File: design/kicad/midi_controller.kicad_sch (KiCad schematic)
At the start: 5 parts, among them J1 Conn_01x16_Socket, J2 Conn_01x25_Socket, J3 Conn_01x25_Socket, U1 CD74HC4067SM

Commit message: Refactor code structure for improved readability and maintainability
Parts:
- removed J1: Conn_01x16_Socket, Connector_PinSocket_2.54mm:PinSocket_1x16_P2.54mm_Vertical, symbol Connector:Conn_01x16_Socket
- removed J2, J3: Conn_01x25_Socket, Connector_PinSocket_2.54mm:PinSocket_1x25_P2.54mm_Vertical, symbol Connector:Conn_01x25_Socket
- removed U1: CD74HC4067SM, Package_SO:SSOP-24_5.3x8.2mm_P0.65mm, symbol 74xx:CD74HC4067SM
- added D1: MIDI_Display_MSP2807, midi_controller:MSP2807_ILI9341_Display, symbol midi_controller:MIDI_Display_MSP2807
- added ENC_MECH1, ENC_MECH2, ENC_MECH3, ENC_MECH4, ENC_MECH5, ENC_MECH6, ENC_MECH7, ENC_MECH8, ENC_MECH9: MIDI_Encoder_PEC11R, midi_controller:PEC11R4220FS0024, symbol midi_controller:MIDI_Encoder_PEC11R
- added ENC_OPT1: MIDI_Encoder_E38S6G5_Optical, midi_controller:E38S6G5_Optical_Encoder, symbol midi_controller:MIDI_Encoder_E38S6G5_Optical
- added J1, J2: Conn_01x24_Socket, symbol Connector:Conn_01x24_Socket
- added R1: R, Resistor_THT:R_Axial_DIN0204_L3.6mm_D1.6mm_P7.62mm_Horizontal, symbol Device:R
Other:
- moved on the sheet: MCU1

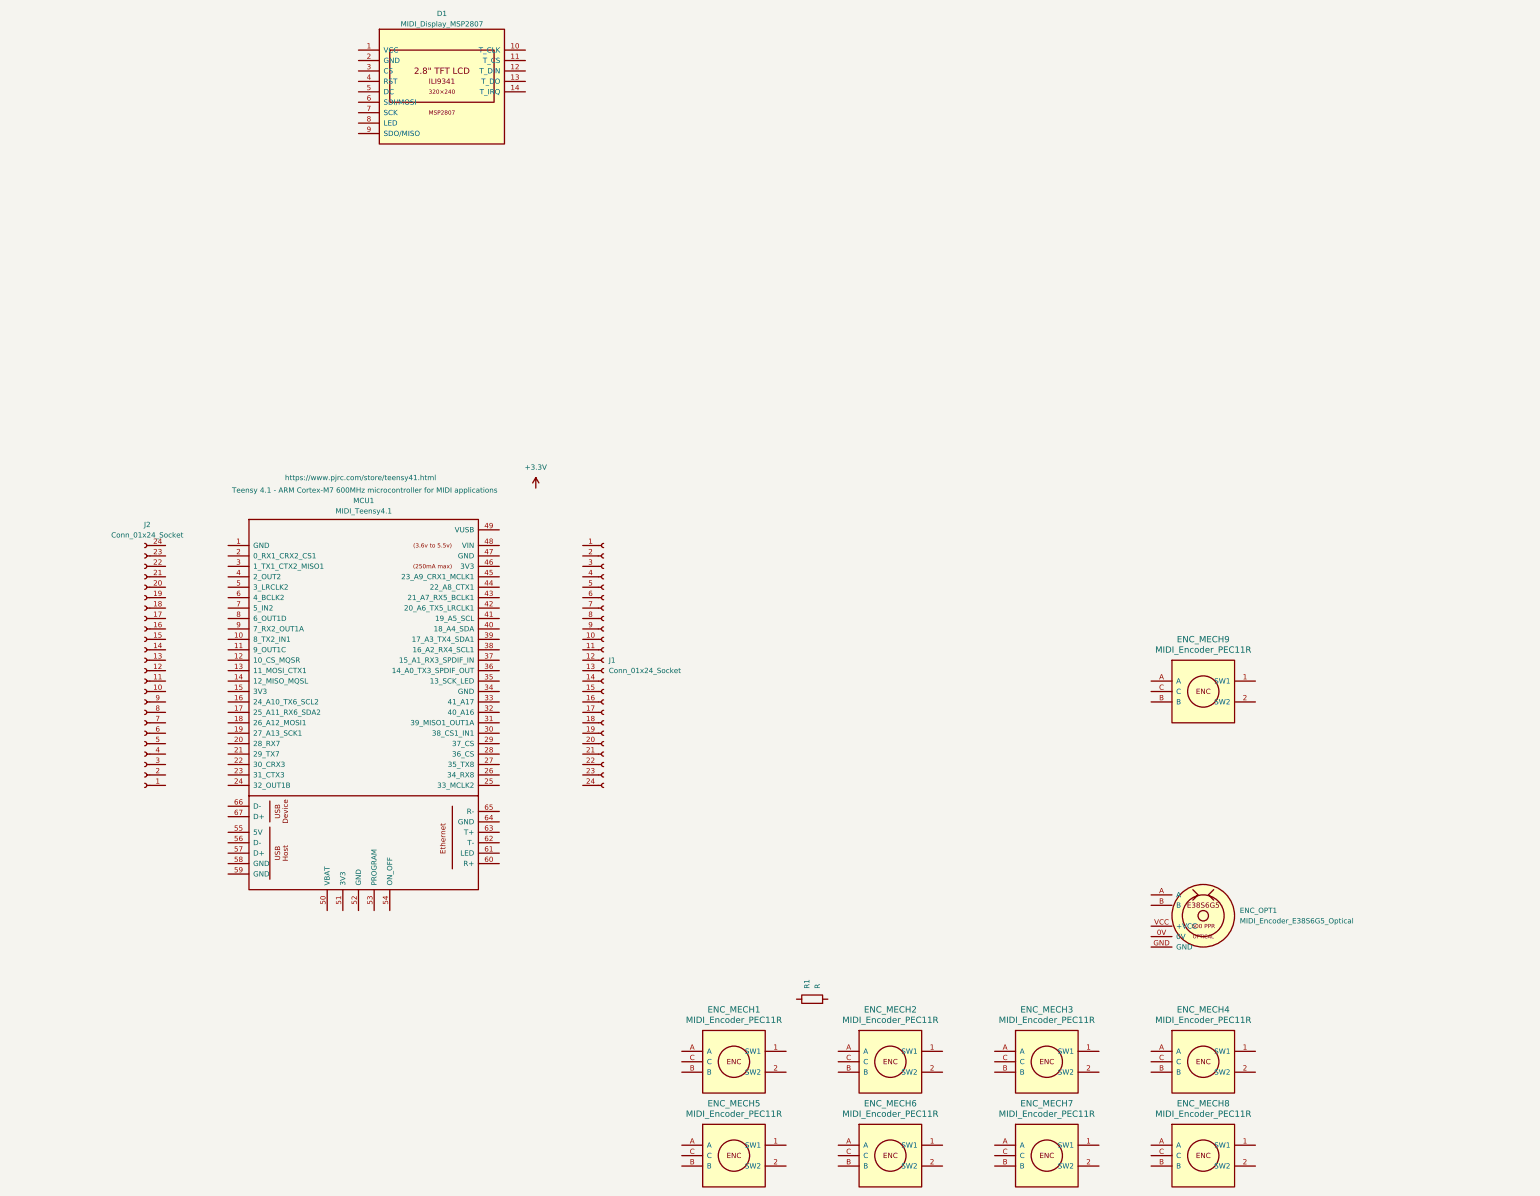
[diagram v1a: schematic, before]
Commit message: Refactor code structure for improved readability and maintainability
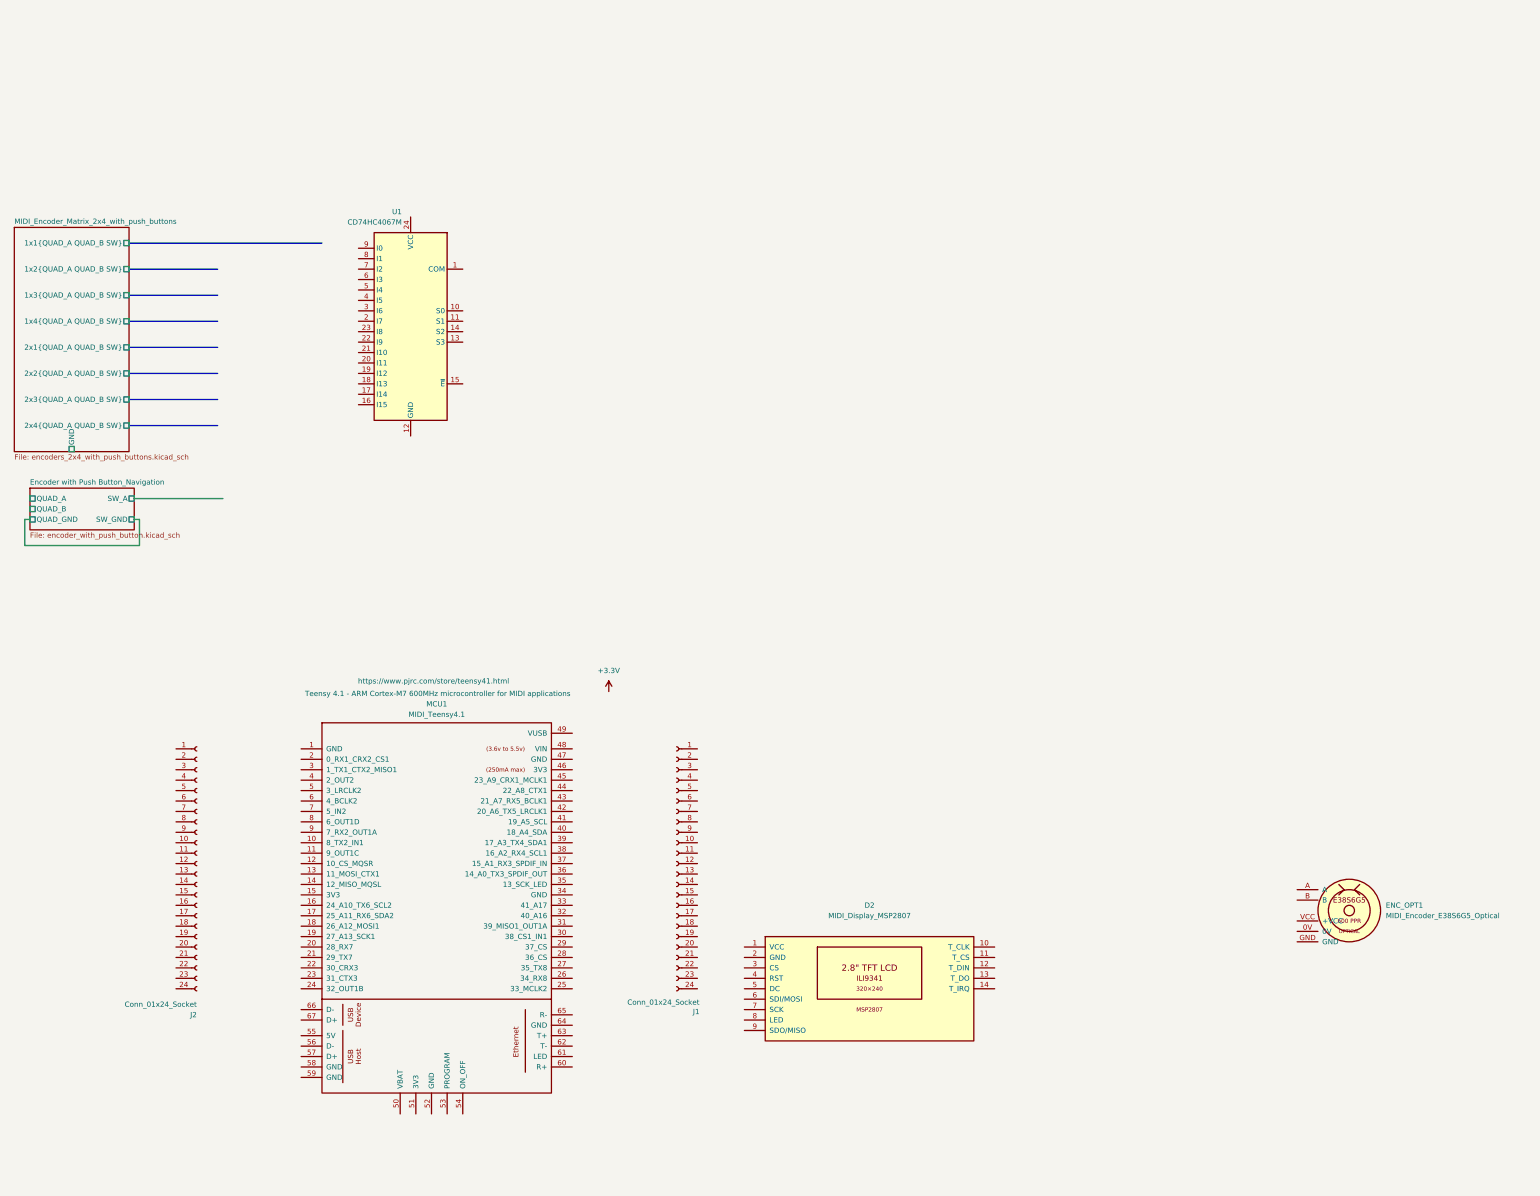
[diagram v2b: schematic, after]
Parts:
- removed D1: MIDI_Display_MSP2807, midi_controller:MSP2807_ILI9341_Display, symbol midi_controller:MIDI_Display_MSP2807
- removed ENC_MECH1, ENC_MECH2, ENC_MECH3, ENC_MECH4, ENC_MECH5, ENC_MECH6, ENC_MECH7, ENC_MECH8, ENC_MECH9: MIDI_Encoder_PEC11R, midi_controller:PEC11R4220FS0024, symbol midi_controller:MIDI_Encoder_PEC11R
- removed R1: R, Resistor_THT:R_Axial_DIN0204_L3.6mm_D1.6mm_P7.62mm_Horizontal, symbol Device:R
- added D2: MIDI_Display_MSP2807, midi_controller:MSP2807_ILI9341_Display, symbol midi_controller:MIDI_Display_MSP2807
- added U1: CD74HC4067M, Package_SO:SSOP-24_5.3x8.2mm_P0.65mm, symbol 74xx:CD74HC4067M
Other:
- added sheet Encoder with Push Button_Navigation (encoder_with_push_button.kicad_sch)
- added sheet MIDI_Encoder_Matrix_2x4_with_push_buttons (encoders_2x4_with_push_buttons.kicad_sch)
- moved on the sheet: ENC_OPT1, J1, J2, MCU1

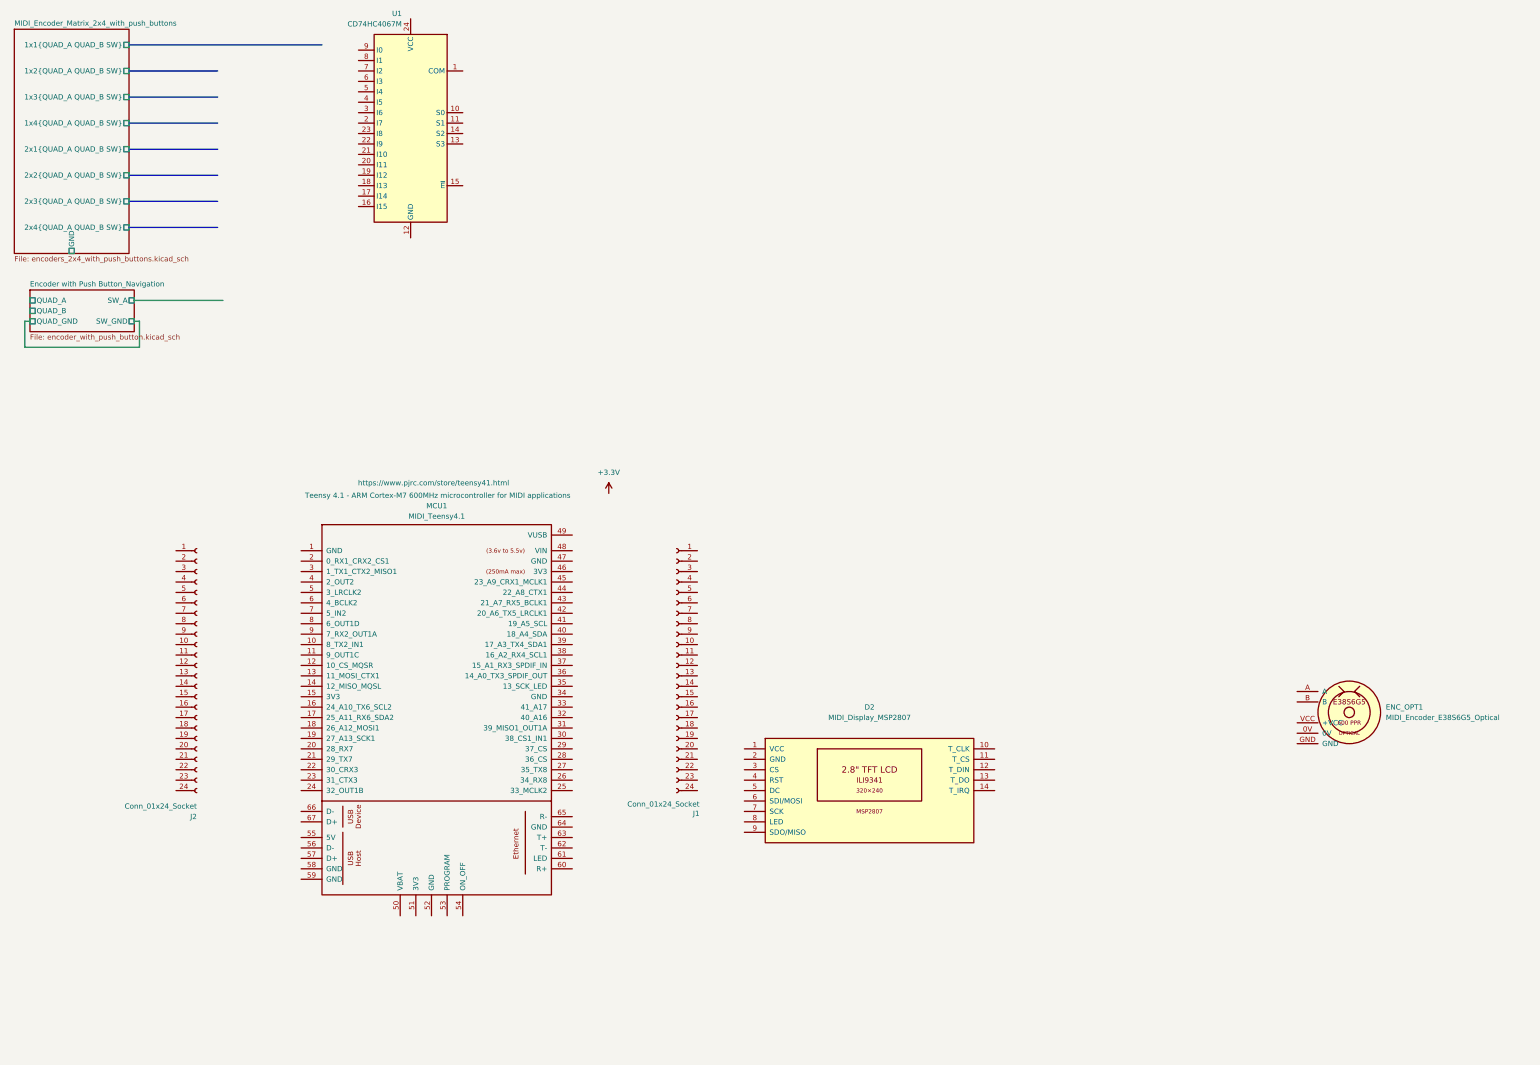
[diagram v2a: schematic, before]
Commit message: Refactor code structure for improved readability and maintainability
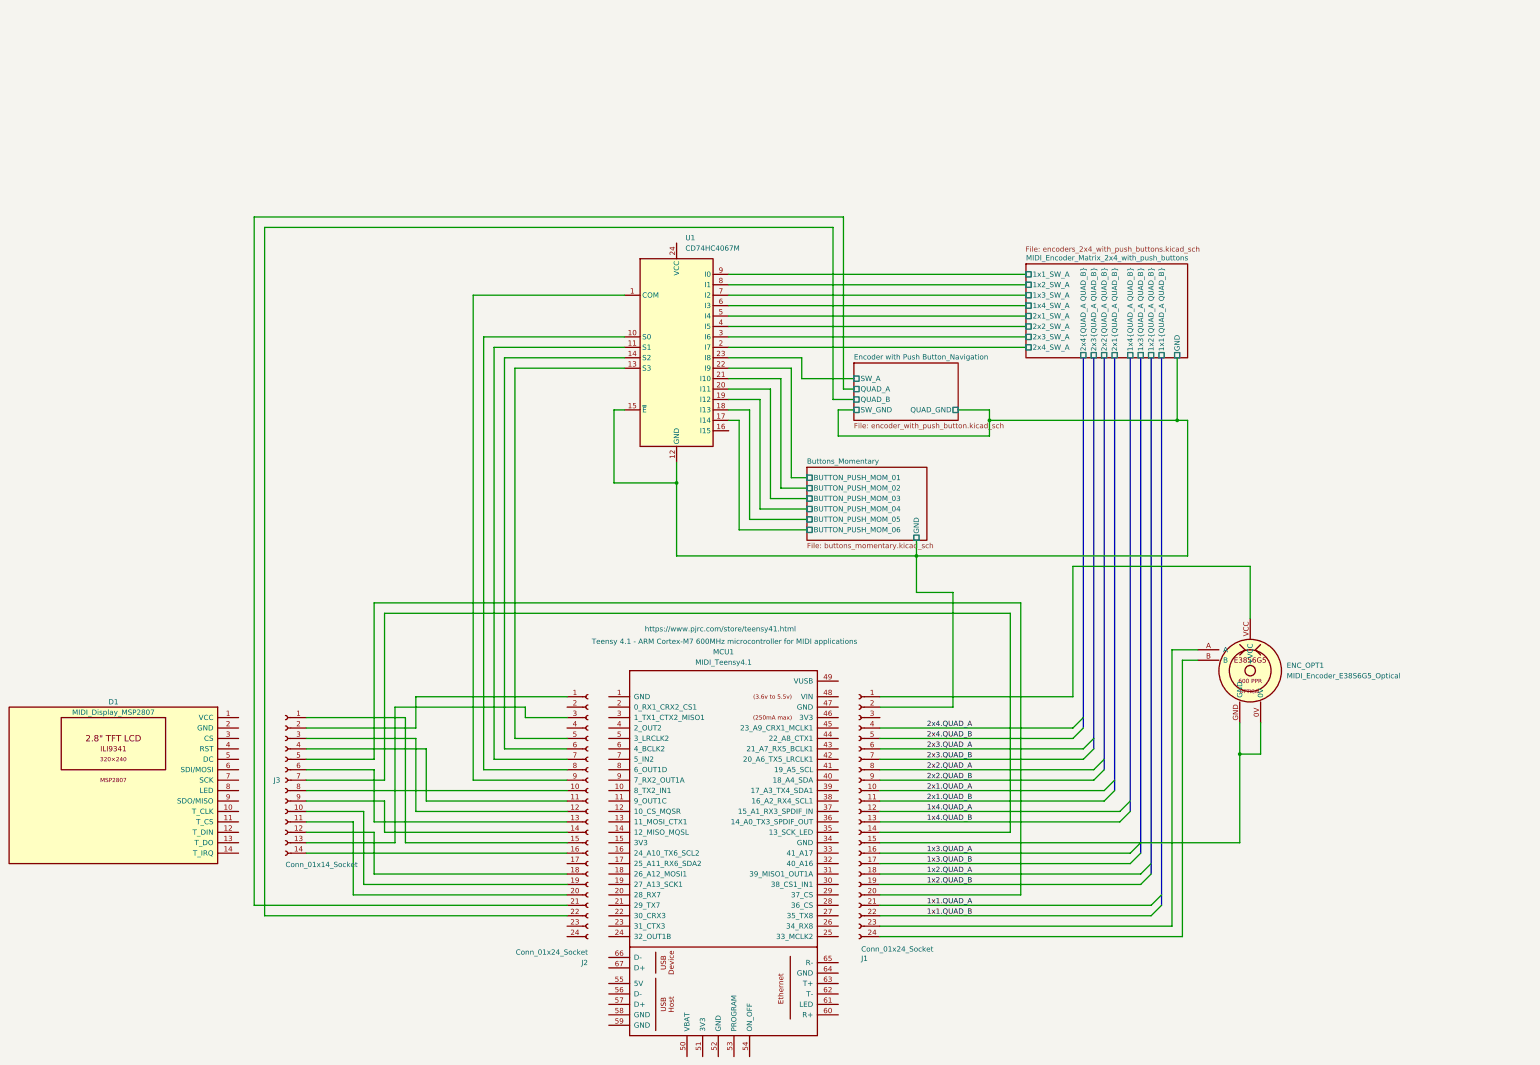
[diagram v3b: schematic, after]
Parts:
- added J3: Conn_01x14_Socket, Connector_PinSocket_2.54mm:PinSocket_1x14_P2.54mm_Vertical, symbol Connector:Conn_01x14_Socket
- J1, J2: footprint (none) -> Connector_PinSocket_2.54mm:PinSocket_1x24_P2.54mm_Vertical
- U1: footprint Package_SO:SSOP-24_5.3x8.2mm_P0.65mm -> Package_SO:SOIC-24W_7.5x15.4mm_P1.27mm
- renumbered D2 to D1
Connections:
- net Encoder with Push Button_Navigation/QUAD_A: now also J2.21 (Pin_21)
- net Encoder with Push Button_Navigation/QUAD_B: now also J2.22 (Pin_22)
- net Encoder with Push Button_Navigation/SW_A: now also U1.23 (I8)
- net at J1.1 (Pin_1): now also ENC_OPT1.VCC (+VCC)
- net 2x1.QUAD_A: now reaches J1.10 (Pin_10)
- net 2x1.QUAD_B: now reaches J1.11 (Pin_11)
- net 1x4.QUAD_A: now reaches J1.12 (Pin_12)
- net 1x4.QUAD_B: now reaches J1.13 (Pin_13)
- net at J1.14 (Pin_14): now also J3.7 (Pin_7)
- net at J1.15 (Pin_15): now also ENC_OPT1.0V, ENC_OPT1.GND
- net 1x3.QUAD_A: now reaches J1.16 (Pin_16)
- net 1x3.QUAD_B: now reaches J1.17 (Pin_17)
- net 1x2.QUAD_A: now reaches J1.18 (Pin_18)
- net 1x2.QUAD_B: now reaches J1.19 (Pin_19)
- net Buttons_Momentary/GND: now reaches J1.2 (Pin_2)
- net Buttons_Momentary/GND: now also U1.12 (GND), U1.15 (~{E})
- net at J1.20 (Pin_20): now also J3.5 (Pin_5)
- net 1x1.QUAD_A: now reaches J1.21 (Pin_21)
- net 1x1.QUAD_B: now reaches J1.22 (Pin_22)
- net at J1.23 (Pin_23): now also ENC_OPT1.A
- net at J1.24 (Pin_24): now also ENC_OPT1.B
- net 2x4.QUAD_A: now reaches J1.4 (Pin_4)
- net 2x4.QUAD_B: now reaches J1.5 (Pin_5)
- net 2x3.QUAD_A: now reaches J1.6 (Pin_6)
- net 2x3.QUAD_B: now reaches J1.7 (Pin_7)
- net 2x2.QUAD_A: now reaches J1.8 (Pin_8)
- net 2x2.QUAD_B: now reaches J1.9 (Pin_9)
- net at U1.1 (COM): now also J2.9 (Pin_9)
- net at U1.10 (S0): now also J2.8 (Pin_8)
- net at U1.11 (S1): now also J2.7 (Pin_7)
- net at U1.13 (S3): now also J2.5 (Pin_5)
- net at U1.14 (S2): now also J2.6 (Pin_6)
- net Buttons_Momentary/BUTTON_PUSH_MOM_06: now reaches U1.17 (I14)
- net Buttons_Momentary/BUTTON_PUSH_MOM_05: now reaches U1.18 (I13)
- net Buttons_Momentary/BUTTON_PUSH_MOM_04: now reaches U1.19 (I12)
- net MIDI_Encoder_Matrix_2x4_with_push_buttons/2x4_SW_A: now reaches U1.2 (I7)
- net Buttons_Momentary/BUTTON_PUSH_MOM_03: now reaches U1.20 (I11)
- net Buttons_Momentary/BUTTON_PUSH_MOM_02: now reaches U1.21 (I10)
- net Buttons_Momentary/BUTTON_PUSH_MOM_01: now reaches U1.22 (I9)
- net MIDI_Encoder_Matrix_2x4_with_push_buttons/2x3_SW_A: now reaches U1.3 (I6)
- net MIDI_Encoder_Matrix_2x4_with_push_buttons/2x2_SW_A: now reaches U1.4 (I5)
- net MIDI_Encoder_Matrix_2x4_with_push_buttons/2x1_SW_A: now reaches U1.5 (I4)
- net MIDI_Encoder_Matrix_2x4_with_push_buttons/1x4_SW_A: now reaches U1.6 (I3)
- net MIDI_Encoder_Matrix_2x4_with_push_buttons/1x3_SW_A: now reaches U1.7 (I2)
- net MIDI_Encoder_Matrix_2x4_with_push_buttons/1x2_SW_A: now reaches U1.8 (I1)
- net MIDI_Encoder_Matrix_2x4_with_push_buttons/1x1_SW_A: now reaches U1.9 (I0)
- net at J2.1 (Pin_1): now also J3.2 (Pin_2)
- net at J2.10 (Pin_10): now also J3.8 (Pin_8)
- net at J2.11 (Pin_11): now also J3.4 (Pin_4)
- net at J2.12 (Pin_12): now also J3.3 (Pin_3)
- net at J2.13 (Pin_13): now also J3.6 (Pin_6)
- net at J2.14 (Pin_14): now also J3.9 (Pin_9)
- net at J2.15 (Pin_15): now also J3.1 (Pin_1)
- net at J2.16 (Pin_16): now also J3.14 (Pin_14)
- net at J2.18 (Pin_18): now also J3.12 (Pin_12)
- net at J2.19 (Pin_19): now also J3.10 (Pin_10)
- net at J2.20 (Pin_20): now also J3.11 (Pin_11)
- net at J2.3 (Pin_3): now also J3.13 (Pin_13)
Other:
- added sheet Buttons_Momentary (buttons_momentary.kicad_sch)
- sheet MIDI_Encoder_Matrix_2x4_with_push_buttons ports: added 1x1_SW_A, 1x1{QUAD_A QUAD_B}, 1x2_SW_A, 1x2{QUAD_A QUAD_B}, 1x3_SW_A, 1x3{QUAD_A QUAD_B}, 1x4_SW_A, 1x4{QUAD_A QUAD_B}, 2x1_SW_A, 2x1{QUAD_A QUAD_B}, 2x2_SW_A, 2x2{QUAD_A QUAD_B}, 2x3_SW_A, 2x3{QUAD_A QUAD_B}, 2x4_SW_A, 2x4{QUAD_A QUAD_B}; removed 1x1{QUAD_A QUAD_B SW}, 1x2{QUAD_A QUAD_B SW}, 1x3{QUAD_A QUAD_B SW}, 1x4{QUAD_A QUAD_B SW}, 2x1{QUAD_A QUAD_B SW}, 2x2{QUAD_A QUAD_B SW}, 2x3{QUAD_A QUAD_B SW}, 2x4{QUAD_A QUAD_B SW}
- moved on the sheet: D1, ENC_OPT1, J1, J2, MCU1, U1
